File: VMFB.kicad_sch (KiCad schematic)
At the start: 123 parts, among them J1 Barrel_Jack_Switch, J10 Conn_01x03_Pin, J11 Conn_01x06_Pin, J12 Conn_01x06_Pin, J13 Conn_01x04_Pin, J14 Conn_01x03_Pin, J15 Conn_01x03_Pin, J17 Conn_01x03_Pin, J18 Conn_01x02_Pin, J2 USB_B, J3 Screw_Terminal_01x02, J4 Screw_Terminal_01x03, J5 Conn_01x03_Pin, J6 Conn_01x03_Pin, J7 Conn_01x03_Pin, J8 Conn_01x04_Pin, J9 Conn_01x02_Pin, Q1 BC547, Q2 BC547, Q3 BC547, Q4 BD139, Q5 TIP41C, Q6 BC547, Q7 BC547, U1 LM358, U2 NE555P, U3 NE555P, U4 NE555P, U5 NE555P

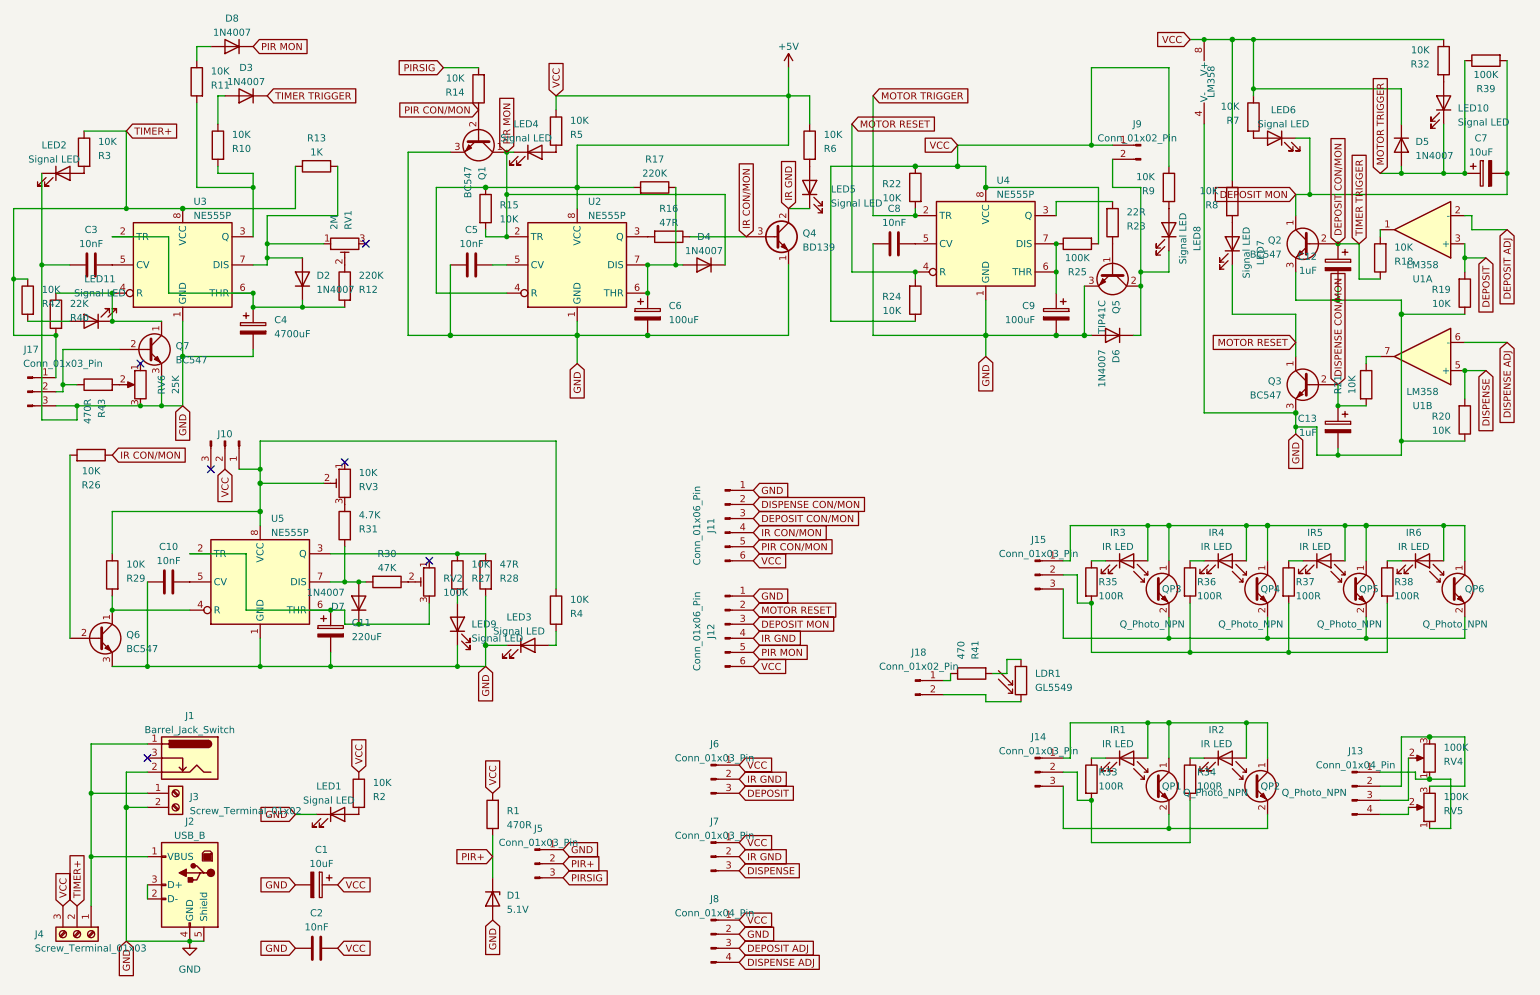
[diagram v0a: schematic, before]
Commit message: more adjustments to the daytimer
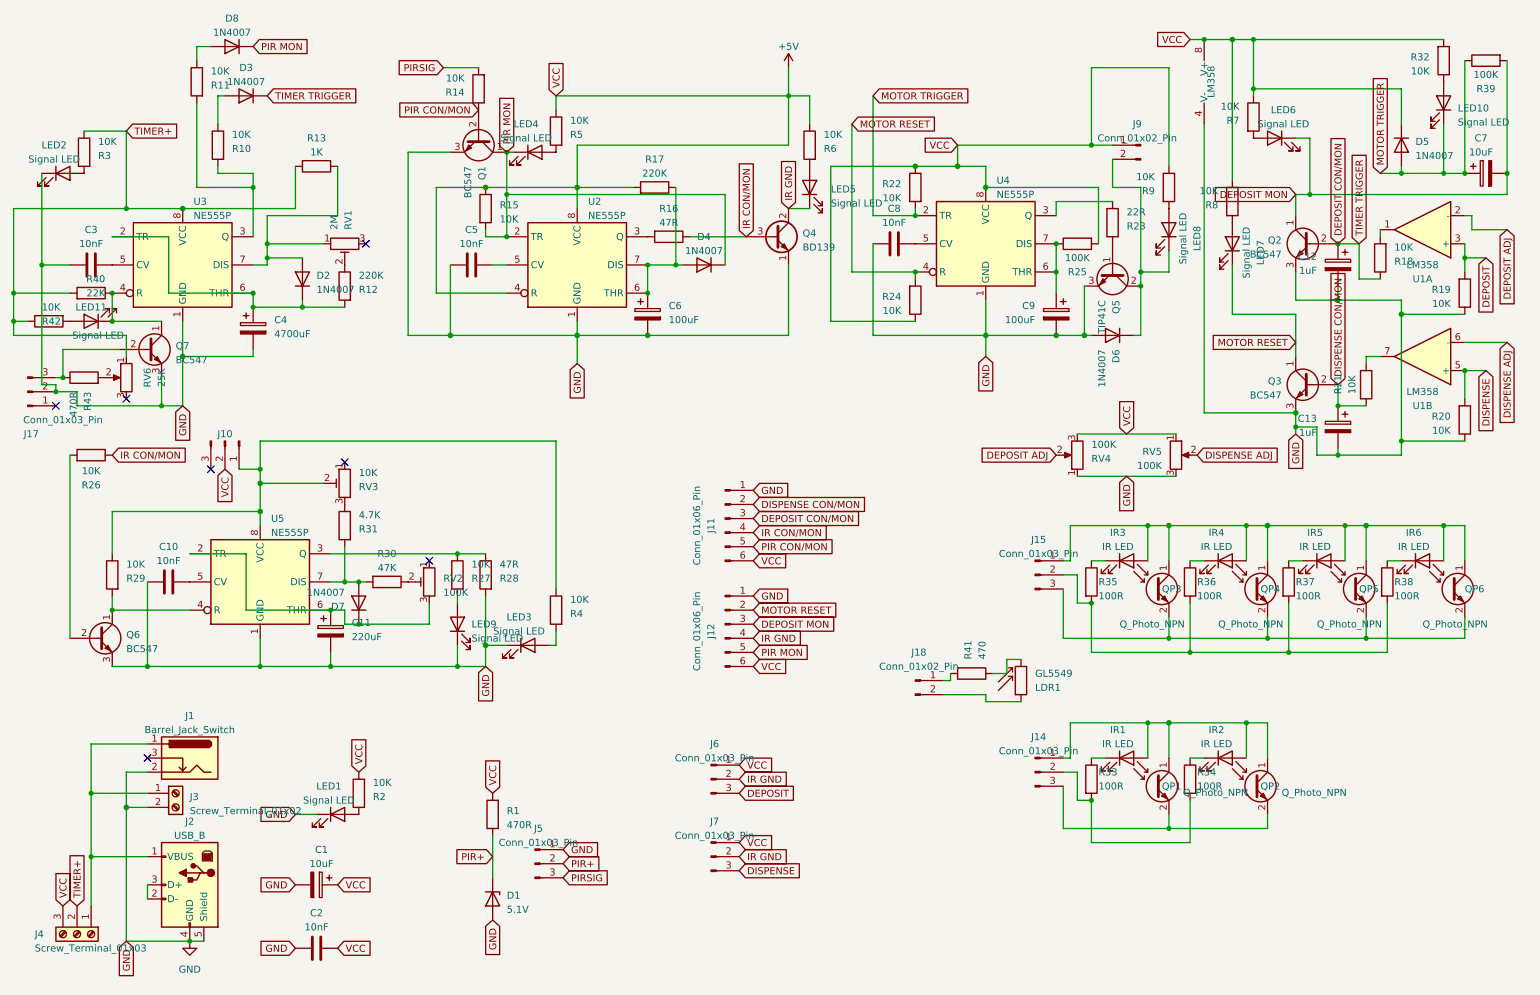
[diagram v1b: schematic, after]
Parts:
- removed J13, J8: Conn_01x04_Pin, Connector_PinHeader_2.54mm:PinHeader_1x04_P2.54mm_Vertical, symbol Connector:Conn_01x04_Pin
- RV4, RV5: footprint Potentiometer_THT:Potentiometer_Piher_T-16H_Single_Horizontal -> Potentiometer_THT:Potentiometer_Piher_PT-10-V10_Vertical
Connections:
- net +5V: now also R32.2, RV4.3, RV5.1; no longer R32.1
- net DEPOSIT ADJ: now also RV4.2
- net DISPENSE ADJ: now also RV5.2
- net GND: now also J17.2 (Pin_2), RV4.1, RV5.3; no longer J17.3 (Pin_3), RV6.3
- net TIMER+: now also RV6.1; no longer J17.1 (Pin_1)
- net at LED10.2 (A): now also R32.1; no longer R32.2
- net at R41.1: now also LDR1.2; no longer J18.1 (Pin_1)
- net at R41.2: now also J18.1 (Pin_1); no longer LDR1.1
- net at Q7.2 (B), R43.1: now also J17.3 (Pin_3); no longer J17.2 (Pin_2)
- net at J18.2 (Pin_2): now also LDR1.1; no longer LDR1.2
- no-connect marks 6 -> 7
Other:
- moved on the sheet: R40, R41, R42, R43, RV4, RV5, RV6
